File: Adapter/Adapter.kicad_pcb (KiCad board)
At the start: 4 copper layers, 20 x 25 mm, 11 parts, among them J2 Conn_01x14_Socket, U1 BGA153 UFS Adapter Modified

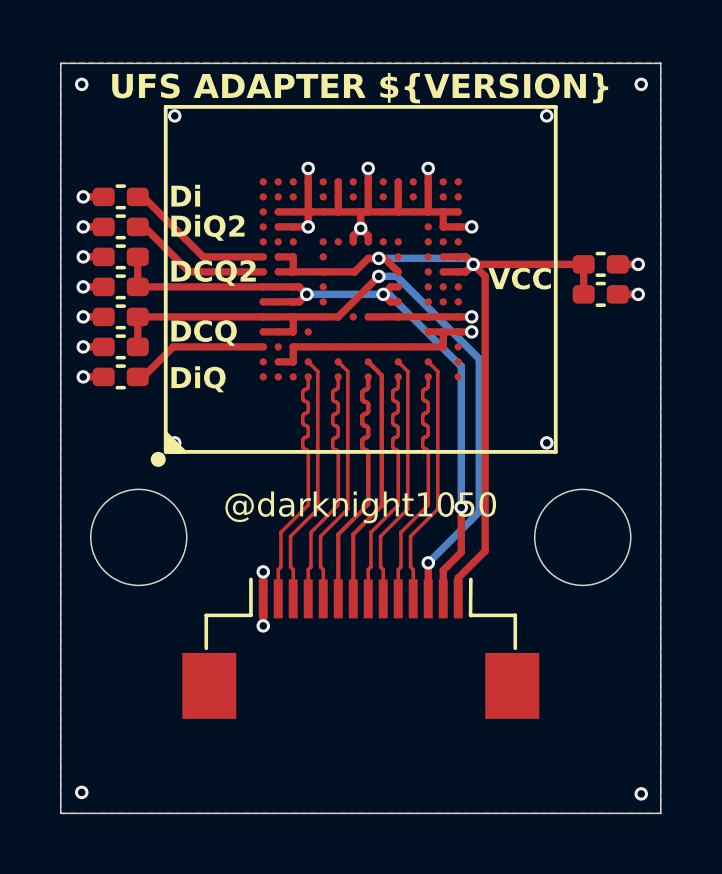
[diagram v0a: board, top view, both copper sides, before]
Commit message: V1.3 GB042 Connector
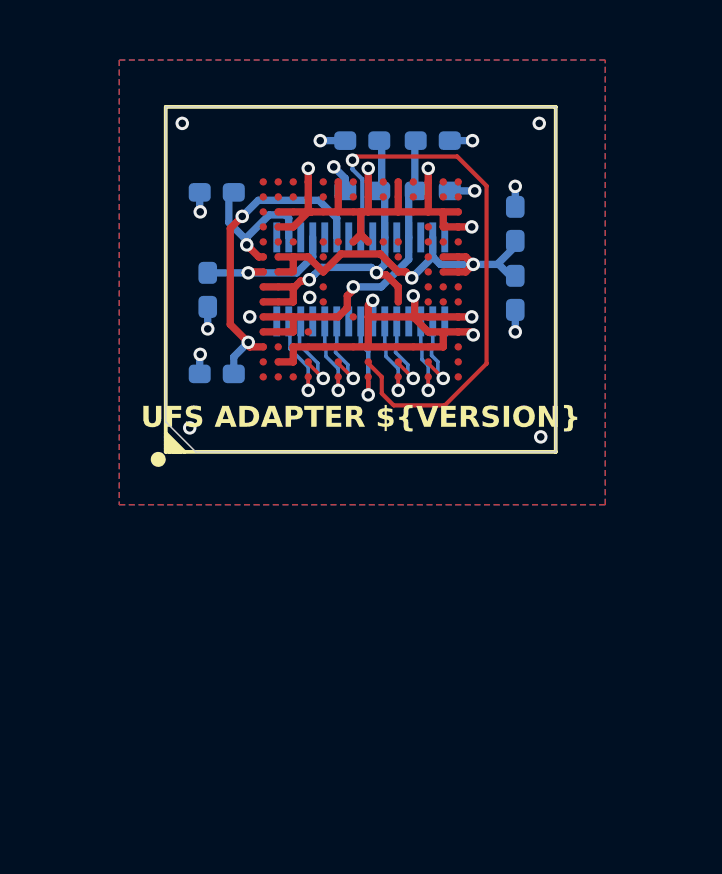
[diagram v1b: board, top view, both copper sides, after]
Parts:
- removed J2: Conn_01x14_Socket, BGA153:FPC 14 Pin 0.5P
- added J1: GB042-30P-H10, BGA153:GB042-30P-H10, B.Cu at (150.0, 90.0)
- C1, C2, C3, C4, C5, C6, C7, C8, C9: moved to B.Cu
- moved C4 11.9 mm to (152.4, 85.4), turned to 0 degrees
- moved C3 11.6 mm to (152.4, 87.0), turned to 0 degrees
- moved C6 9.41 mm to (150.1, 85.4)
- moved C5 8.35 mm to (150.1, 87.0)
- moved C9 3.58 mm to (144.9, 90.3), turned to -90 degrees
- moved C7 3.20 mm to (145.2, 87.1)
- moved C8 3.20 mm to (145.2, 93.2)
- moved C2 3.15 mm to (155.2, 88.2), turned to 90 degrees
- moved C1 2.85 mm to (155.2, 90.5), turned to -90 degrees
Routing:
- net VCC: track 27.2 -> 14.0 mm
- net VCCQ: track 24.3 -> 11.4 mm, vias 2 -> 1
- net VCCQ2: track 23.6 -> 11.6 mm, vias 3 -> 2
- net /RST_N: track 8.48 -> 19.3 mm, vias 0 -> 1
- net /VDDiQ: track 4.60 -> 10.7 mm, vias 0 -> 2
- net /RX1P: track 8.45 -> 2.84 mm, vias 0 -> 1
- net /RX1N: track 8.40 -> 2.85 mm, vias 0 -> 1
- net /RX0P: track 8.45 -> 2.92 mm, vias 0 -> 1
- net /TX0N: track 8.45 -> 2.92 mm, vias 0 -> 1
- net /RX0N: track 8.40 -> 2.94 mm, vias 0 -> 1
- net /TX0P: track 8.40 -> 2.94 mm, vias 0 -> 1
- net /TX1N: track 8.45 -> 3.00 mm, vias 0 -> 1
- net /TX1P: track 8.40 -> 3.02 mm, vias 0 -> 1
- net /REF_CLK: track 8.45 -> 3.15 mm, vias 0 -> 1
- net VSS: track 36.3 -> 38.3 mm, vias 27 -> 23
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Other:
- board size 20 x 25 mm -> 13 x 11.5 mm
